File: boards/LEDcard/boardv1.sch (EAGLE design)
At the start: 38 parts, among them K1 NA, K2 NA, K3 NA, K4 NA, K5 NA, K6 NA, X1 112404, X2 112404, X3 112404, X4 112404, X5 112404, X6 112404, X7 112404, X8 112404

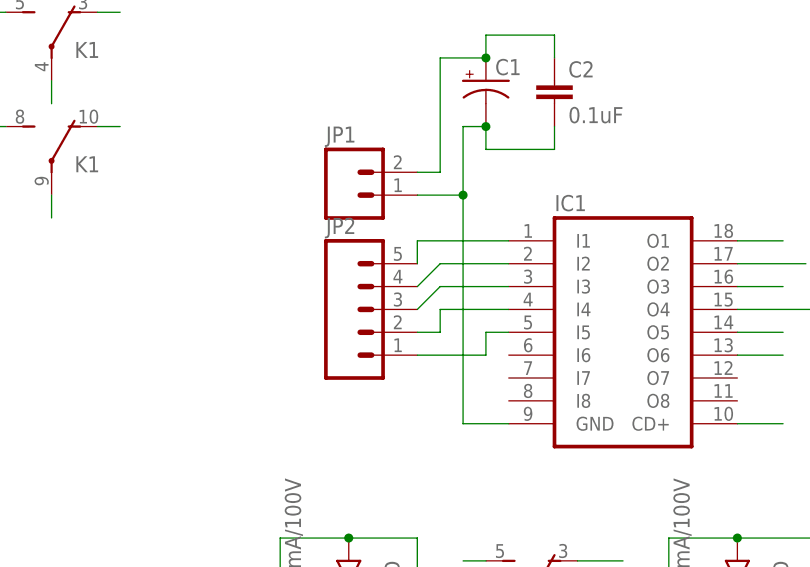
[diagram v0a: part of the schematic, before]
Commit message: Board update
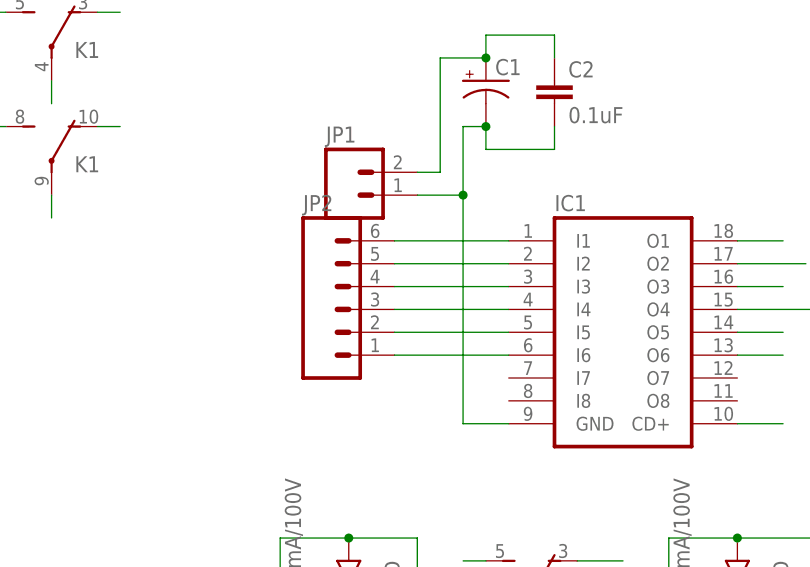
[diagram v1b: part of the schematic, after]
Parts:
- C2: device SparkFun-Capacitors:0.1UF-50V-20%(PTH)KIT-EZ -> SparkFun-Capacitors:0.1UF-25V-5%(0603)
- JP2: device SparkFun-Connectors:M05PTH -> SparkFun-Connectors:M06NO_SILK_YES_STOP
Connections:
- removed net N$21: IC1.I1, JP2.5
- removed net N$22: IC1.I2, JP2.4
- removed net N$23: IC1.I3, JP2.3
- new net GND2: C1.-, C2.2, IC1.GND, JP1.1
- new net N$10: IC1.I2, JP2.5
- new net N$11: IC1.I3, JP2.4
- new net N$8: IC1.I6, JP2.1
- new net N$9: IC1.I1, JP2.6
- net GND: no longer C1.-, C2.2, IC1.GND, JP1.1
- net N$24: now also JP2.3; no longer JP2.2
- net N$25: now also JP2.2; no longer JP2.1
